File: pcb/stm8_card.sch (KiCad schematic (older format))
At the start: 25 parts, among them J1 DEBUG HEADER, SW1 TL59AF100Q, SW2 TL59AF100Q, SW3 TL59AF100Q, SW4 TL3302AF260QG, U1 ER-OLED0.91-7, U2 STM8S103F3

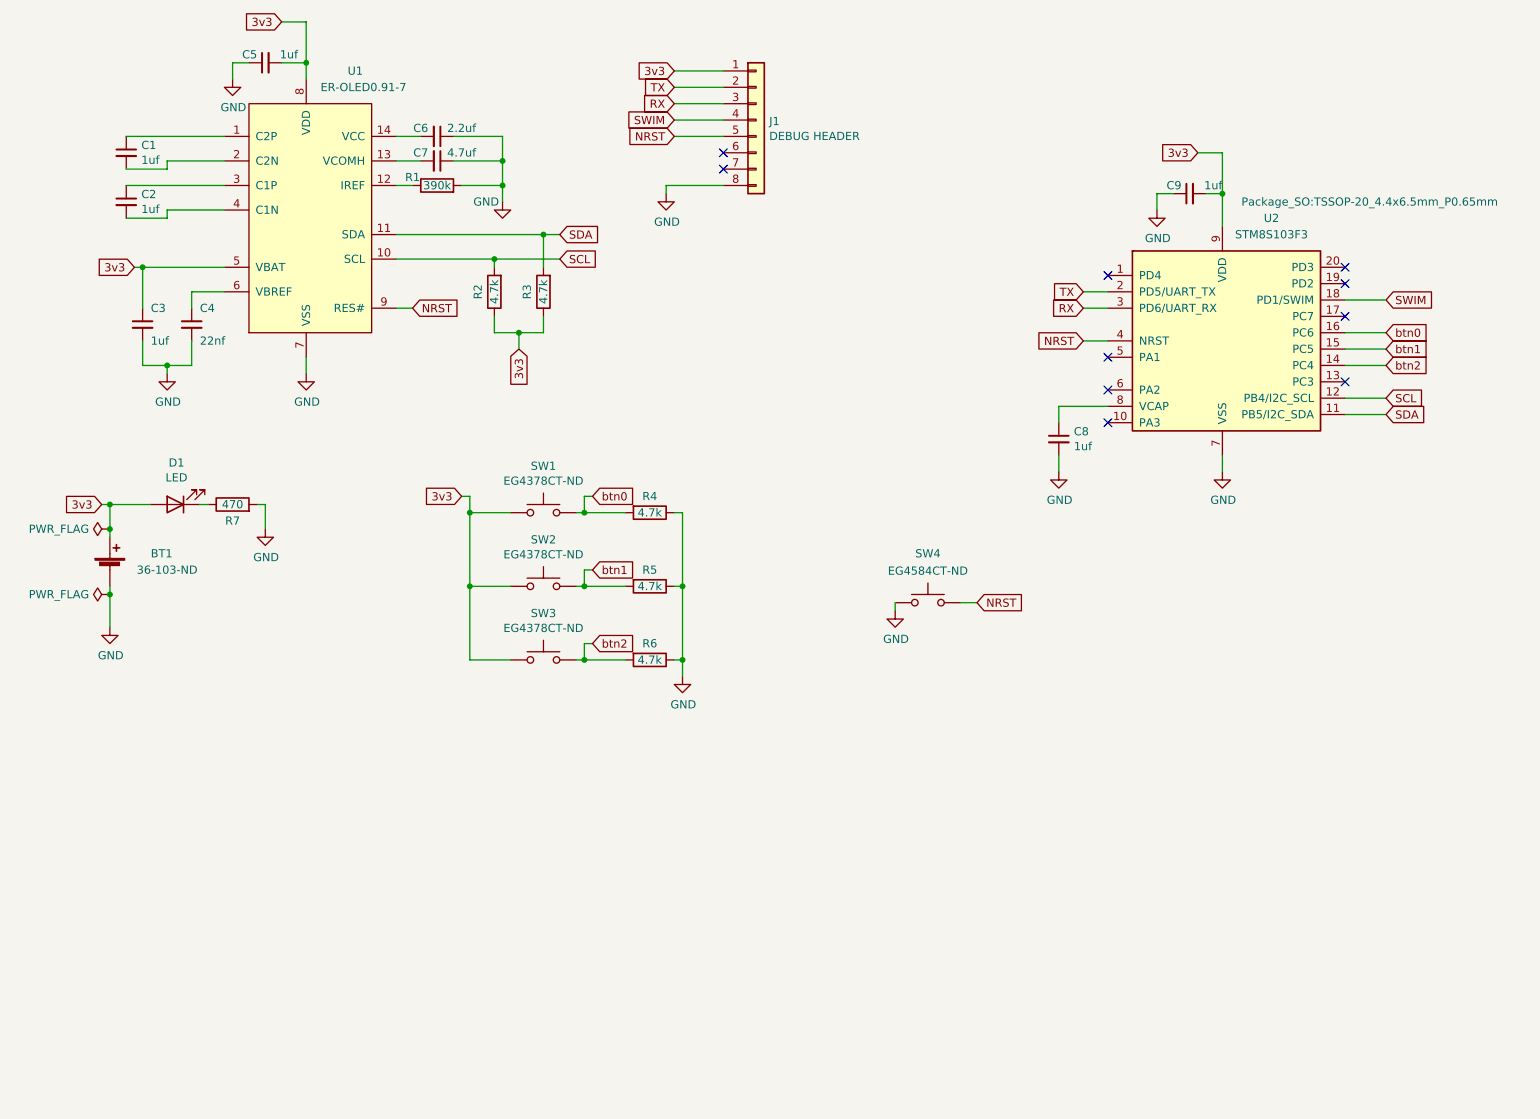
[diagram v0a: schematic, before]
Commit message: rough schematic update
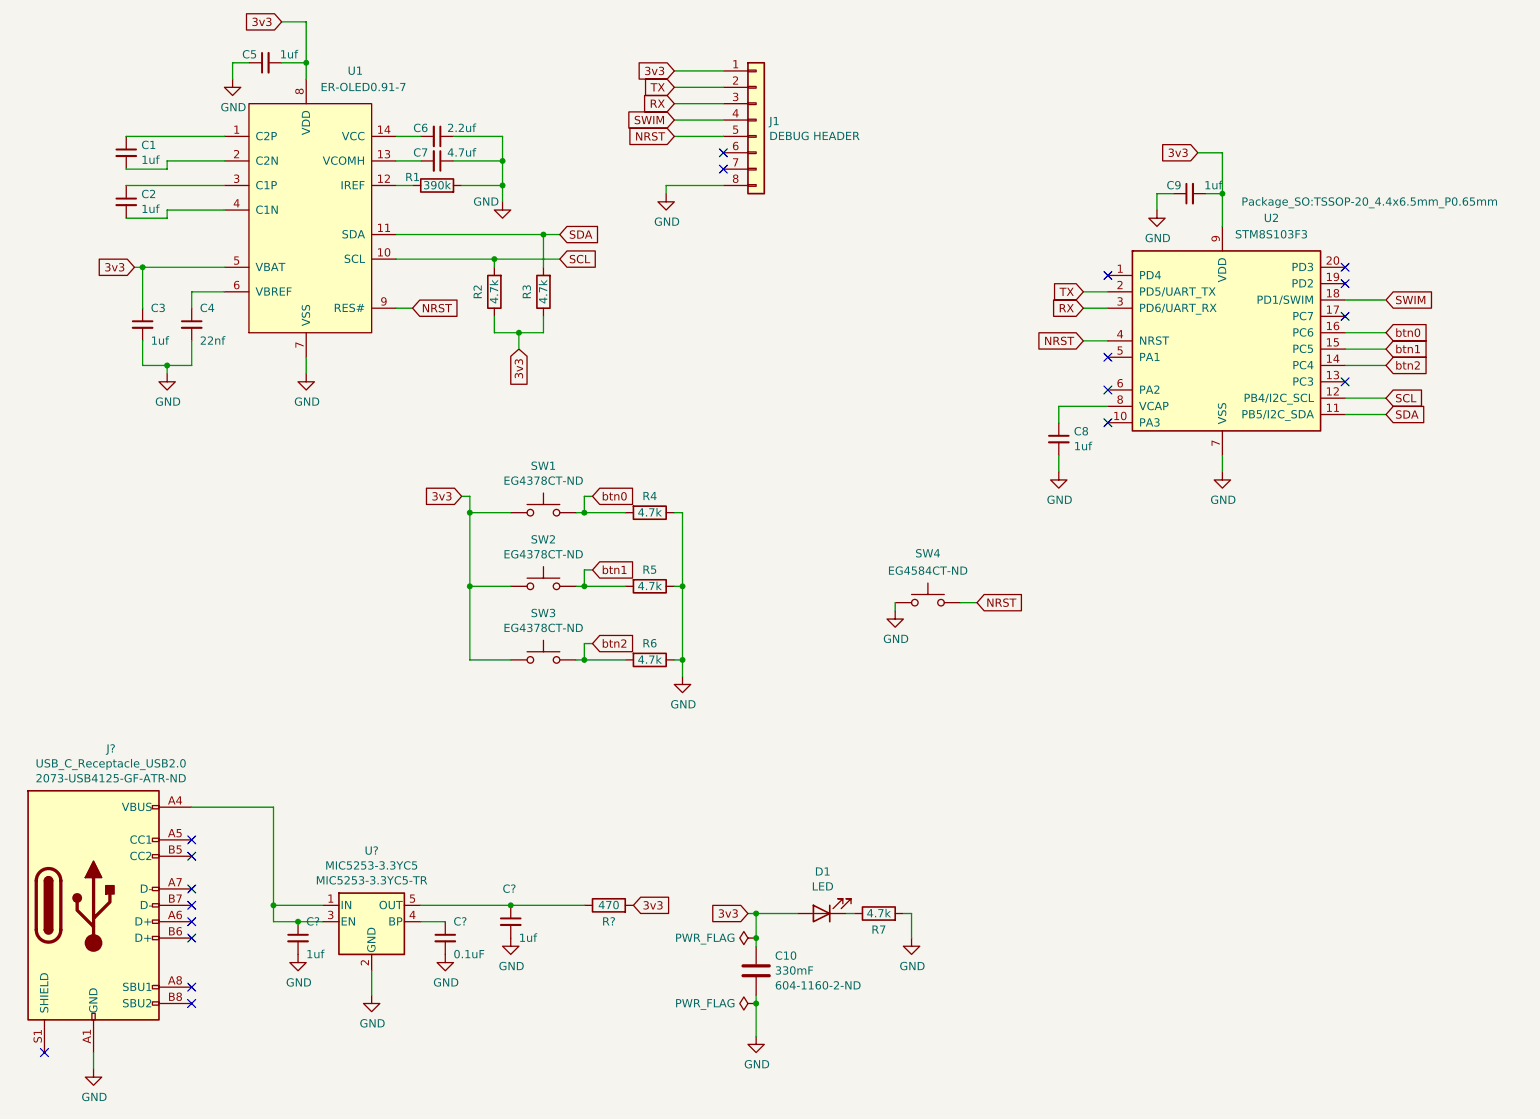
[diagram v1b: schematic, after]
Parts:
- removed BT1: 103, stm8_card:BatteryHolder_Keystone_103_1x20mm_Corrected, symbol stm8_card-rescue:Battery_Cell-Device
- added C10: 330mF, symbol Device:C
- added C? (x2): 1uf, Capacitor_SMD:C_0805_2012Metric_Pad1.18x1.45mm_HandSolder, symbol stm8_card-rescue:C_Small-Device
- added C?: 0.1uF, Capacitor_SMD:C_0805_2012Metric_Pad1.18x1.45mm_HandSolder, symbol stm8_card-rescue:C_Small-Device
- added J?: USB_C_Receptacle_USB2.0, symbol Connector:USB_C_Receptacle_USB2.0
- added R?: 470, Resistor_SMD:R_0805_2012Metric_Pad1.20x1.40mm_HandSolder, symbol stm8_card-rescue:R-Device
- added U?: MIC5253-3.3YC5, Package_TO_SOT_SMD:SOT-23-5, symbol Regulator_Linear:MIC5205-3.3YM5
- R7: value 470 -> 4.7k
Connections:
- net 3v3: now also C10.1, R?.2
- net GND: now also C10.2, C?.2, C?.2, C?.2, J?.A1 (GND), J?.A12 (GND), J?.B1 (GND), J?.B12 (GND), U?.2 (GND)
- new net: C?.1, J?.A4 (VBUS), J?.A9 (VBUS), J?.B4 (VBUS), J?.B9 (VBUS), U?.1 (IN), U?.3 (EN)
- new net: C?.1, U?.4 (BP)
- new net: C?.1, R?.1, U?.5 (OUT)
- no-connect marks 10 -> 19
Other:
- moved on the sheet: D1, R7
